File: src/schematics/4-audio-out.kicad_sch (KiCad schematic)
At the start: 34 parts, among them U401 AP22653AW6, U402 MCP6486U, U403 IS31AP4991A-SLS2

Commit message: Started to lay out the PCB.
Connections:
- net GND_PWRIN renamed GND

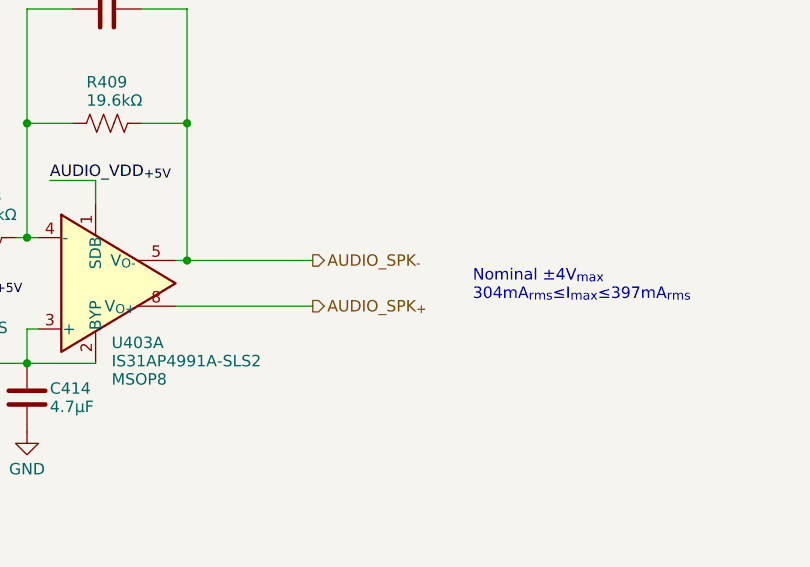
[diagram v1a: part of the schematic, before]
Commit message: PCB routing.
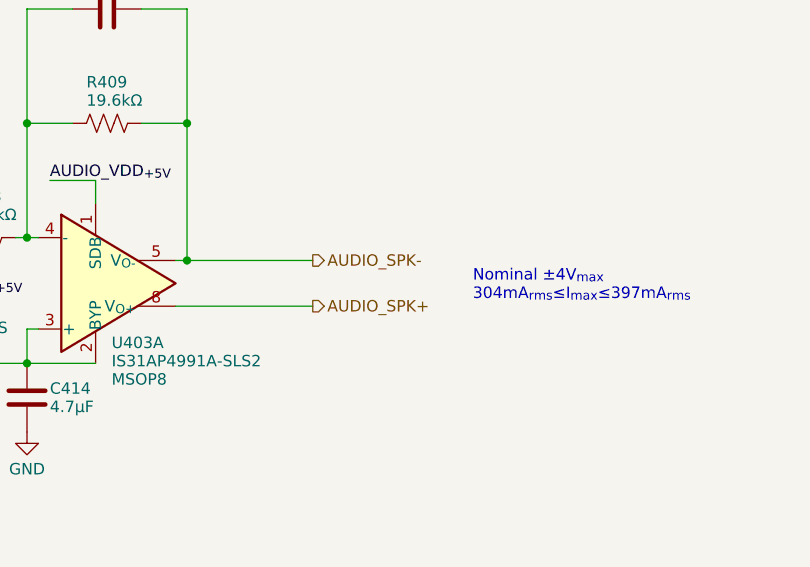
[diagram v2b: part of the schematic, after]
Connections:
- net AUDIO_SPK_{+} renamed AUDIO_SPK+
- net AUDIO_SPK_{-} renamed AUDIO_SPK-
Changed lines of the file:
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@@
     (effects (font (size 1.27 1.27)) (justify right))
   )
-  (hierarchical_label "AUDIO_SPK_{+}" (shape output) (at 266.7 160.02 0) (fields_autoplaced)
+  (hierarchical_label "AUDIO_SPK+" (shape output) (at 266.7 160.02 0) (fields_autoplaced)
     (effects (font (size 1.27 1.27)) (justify left))
   )
-  (hierarchical_label "AUDIO_SPK_{-}" (shape output) (at 266.7 154.94 0) (fields_autoplaced)
+  (hierarchical_label "AUDIO_SPK-" (shape output) (at 266.7 154.94 0) (fields_autoplaced)
     (effects (font (size 1.27 1.27)) (justify left))
   )
